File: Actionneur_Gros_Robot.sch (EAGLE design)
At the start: 52 parts, among them M1 ARDUINO-NANO-3.0, M10 SERVO, M11 SERVO, M2 SERVO, M3 SERVO, M4 SERVO, M5 SERVO, M6 SERVO, M7 SERVO, M8 SERVO, M9 SERVO, Y1 16MHz

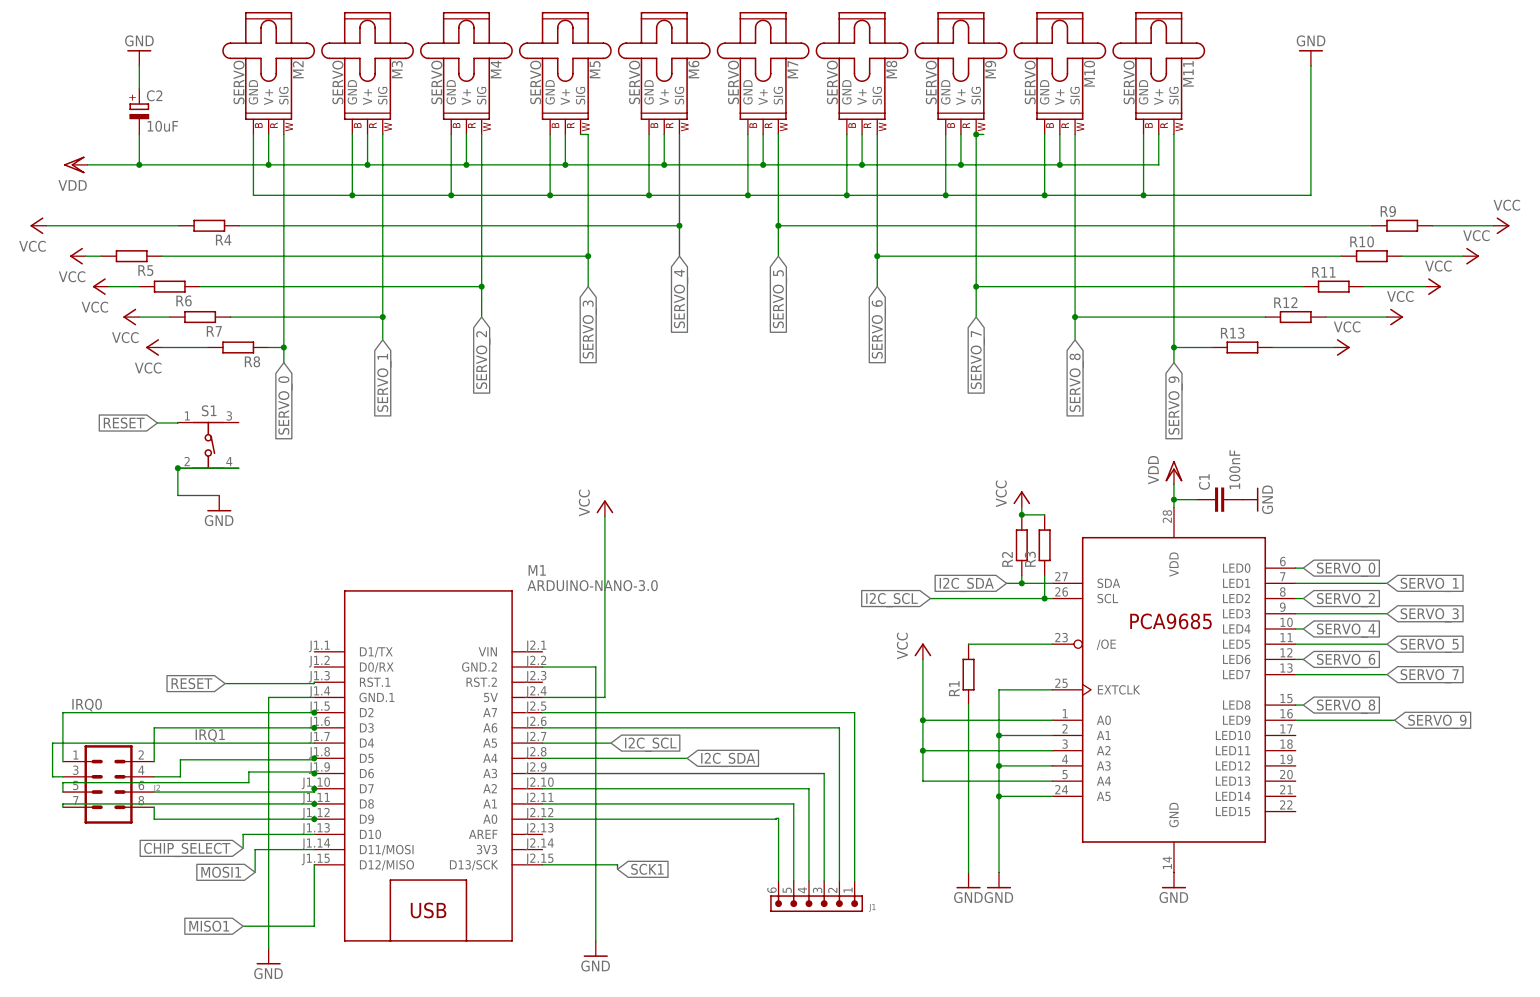
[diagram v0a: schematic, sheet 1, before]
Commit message: revA02
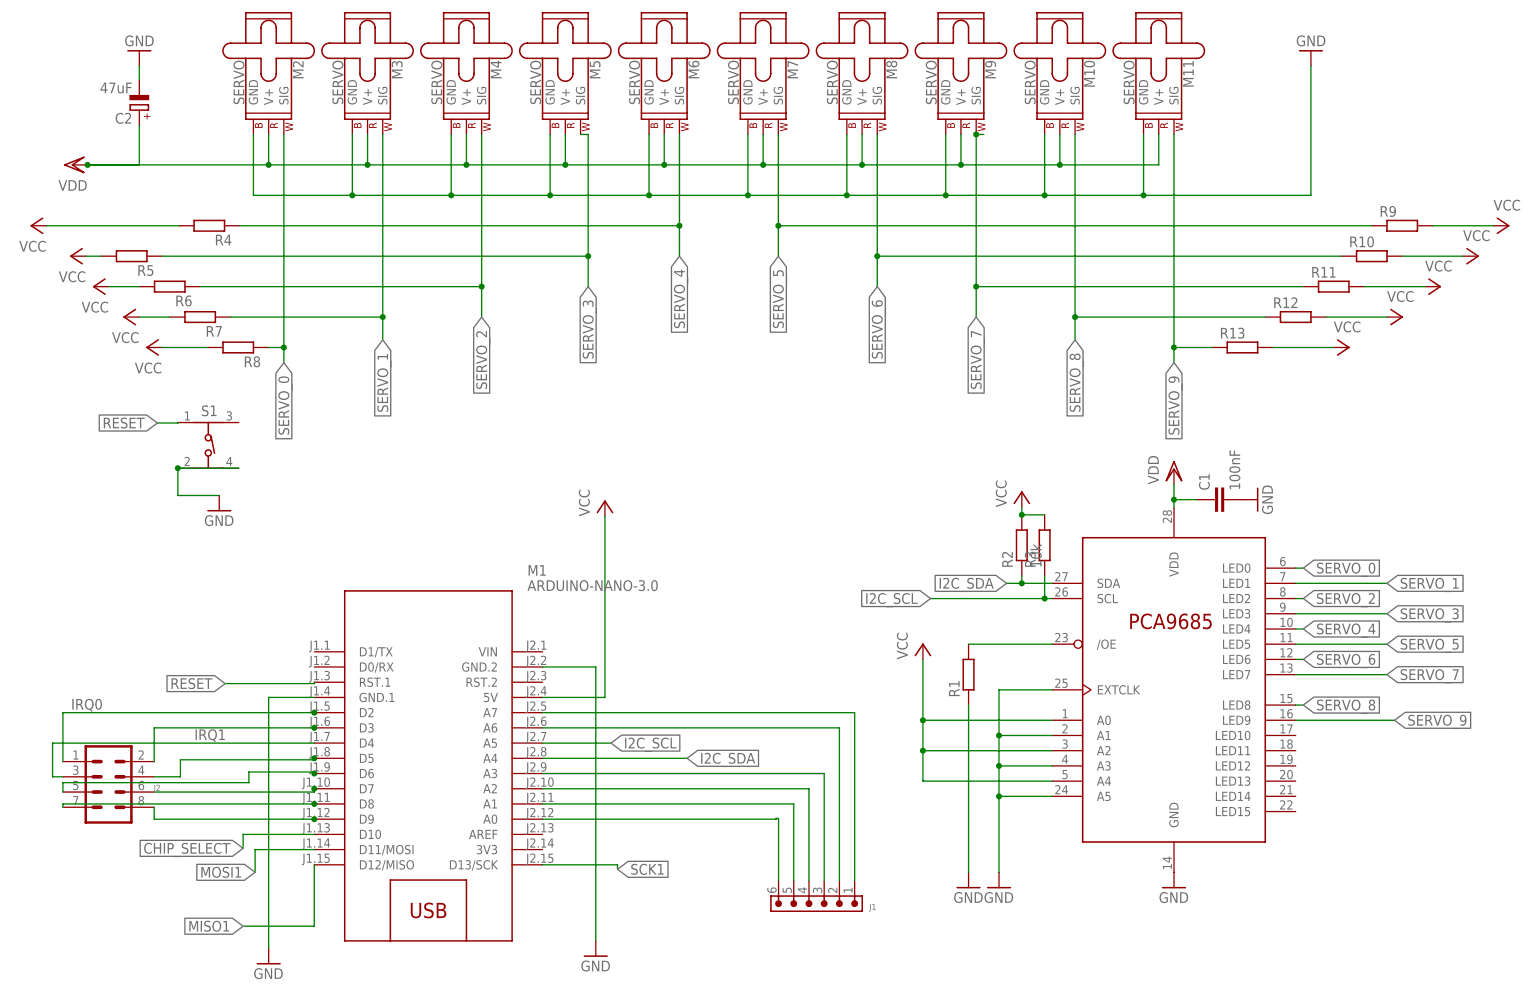
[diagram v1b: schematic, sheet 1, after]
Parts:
- C2: value 10uF -> 47uF
- R2: value (none) -> 10k
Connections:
- net GND: now also C2.-; no longer C2.+
- net VDD: now also C2.+; no longer C2.-
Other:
- moved on the sheet: C2
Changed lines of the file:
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@@
 <part name="C1" library="rcl" library_urn="urn:adsk.eagle:library:334" deviceset="C-EU" device="025-025X050" package3d_urn="urn:adsk.eagle:package:23629/2" value="100nF"/>
 <part name="GND4" library="supply1" library_urn="urn:adsk.eagle:library:371" deviceset="GND" device=""/>
-<part name="R2" library="rcl" library_urn="urn:adsk.eagle:library:334" deviceset="R-EU_" device="0204/7" package3d_urn="urn:adsk.eagle:package:23498/2"/>
+<part name="R2" library="rcl" library_urn="urn:adsk.eagle:library:334" deviceset="R-EU_" device="0204/7" package3d_urn="urn:adsk.eagle:package:23498/2" value="10k"/>
 <part name="R3" library="rcl" library_urn="urn:adsk.eagle:library:334" deviceset="R-EU_" device="0204/7" package3d_urn="urn:adsk.eagle:package:23498/2"/>
 <part name="P+2" library="supply1" library_urn="urn:adsk.eagle:library:371" deviceset="VCC" device=""/>
@@
 <part name="VDD9" library="supply1" library_urn="urn:adsk.eagle:library:371" deviceset="VDD" device=""/>
 <part name="GND17" library="supply1" library_urn="urn:adsk.eagle:library:371" deviceset="GND" device=""/>
-<part name="C2" library="rcl" library_urn="urn:adsk.eagle:library:334" deviceset="CPOL-EU" device="E2.5-7" package3d_urn="urn:adsk.eagle:package:23345/1" value="10uF"/>
+<part name="C2" library="rcl" library_urn="urn:adsk.eagle:library:334" deviceset="CPOL-EU" device="E2.5-7" package3d_urn="urn:adsk.eagle:package:23345/1" value="47uF"/>
 <part name="C5" library="rcl" library_urn="urn:adsk.eagle:library:334" deviceset="C-EU" device="025-025X050" package3d_urn="urn:adsk.eagle:package:23629/2" value="100nF"/>
 <part name="VDD10" library="supply1" library_urn="urn:adsk.eagle:library:371" deviceset="VDD" device=""/>
@@
 <attribute name="VALUE" x="37.48" y="88.322" size="1.778" layer="96"/>
 </instance>
-<instance part="C2" gate="G$1" x="26.67" y="158.75" smashed="yes">
-<attribute name="NAME" x="27.813" y="159.2326" size="1.778" layer="95"/>
-<attribute name="VALUE" x="27.813" y="154.1526" size="1.778" layer="96"/>
+<instance part="C2" gate="G$1" x="26.67" y="157.734" smashed="yes" rot="R180">
+<attribute name="NAME" x="25.527" y="157.2514" size="1.778" layer="95" rot="R180"/>
+<attribute name="VALUE" x="25.527" y="162.3314" size="1.778" layer="96" rot="R180"/>
 </instance>
 <instance part="P+4" gate="VCC" x="104.394" y="92.456" smashed="yes">
@@
 </segment>
 <segment>
-<pinref part="C2" gate="G$1" pin="+"/>
 <pinref part="GND8" gate="1" pin="GND"/>
-<wire x1="26.67" y1="161.29" x2="26.67" y2="165.1" width="0.1524" layer="91"/>
+<pinref part="C2" gate="G$1" pin="-"/>
+<wire x1="26.67" y1="165.1" x2="26.67" y2="162.814" width="0.1524" layer="91"/>
 </segment>
 </net>
@@
 <net name="VDD" class="0">
 <segment>
-<pinref part="C2" gate="G$1" pin="-"/>
-<wire x1="26.67" y1="153.67" x2="26.67" y2="148.59" width="0.1524" layer="91"/>
 <pinref part="P+5" gate="G$1" pin="VDD"/>
-<wire x1="18.034" y1="148.59" x2="26.67" y2="148.59" width="0.1524" layer="91"/>
 <pinref part="M2" gate="G$1" pin="V+"/>
 <wire x1="48.26" y1="153.67" x2="48.26" y2="148.59" width="0.1524" layer="91"/>
-<wire x1="26.67" y1="148.59" x2="48.26" y2="148.59" width="0.1524" layer="91"/>
-<junction x="26.67" y="148.59"/>
+<wire x1="18.034" y1="148.59" x2="48.26" y2="148.59" width="0.1524" layer="91"/>
 <pinref part="M3" gate="G$1" pin="V+"/>
 <wire x1="64.77" y1="153.67" x2="64.77" y2="148.59" width="0.1524" layer="91"/>
@@
 <wire x1="180.34" y1="148.59" x2="196.85" y2="148.59" width="0.1524" layer="91"/>
 <junction x="180.34" y="148.59"/>
-</segment>
-</net>
+<pinref part="C2" gate="G$1" pin="+"/>
+<wire x1="26.67" y1="155.194" x2="26.67" y2="148.59" width="0.1524" layer="91"/>
+<wire x1="26.67" y1="148.59" x2="18.034" y2="148.59" width="0.1524" layer="91"/>
+<junction x="18.034" y="148.59"/>
+</segment>
+</net>
